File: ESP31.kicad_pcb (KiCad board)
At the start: 4 copper layers, 20.7 x 37.3 mm, 51 parts, among them J1 Conn_01x01, J25 Conn_01x01, J26 Conn_01x01, J27 Conn_01x01, J28 Conn_01x01, J29 Conn_01x01, J30 Conn_01x01, J31 Conn_01x01, J32 Conn_01x01, J33 Conn_01x01, J34 Conn_01x01, J35 Conn_01x01, J36 Conn_01x01, J40 Conn_01x01, J41 Conn_01x01, J42 Conn_01x01, J43 Conn_01x01, J44 Conn_01x01, J45 Conn_01x01, J46 Conn_01x01, J47 Conn_01x01, J48 Conn_01x01, J49 Conn_01x01, J50 Conn_01x01, J51 Conn_01x01, J52 Conn_01x01, J53 Conn_01x01, J54 Conn_01x01, J55 Conn_01x01, J56 Conn_01x01, J57 Conn_01x01, J58 Conn_01x01, J59 Conn_01x01, J60 Conn_01x01, J61 Conn_01x01, J62 Conn_01x01, J63 Conn_01x01, SW1 SW_Push, SW2 SW_Push, U1 ESP32-PICO-D4

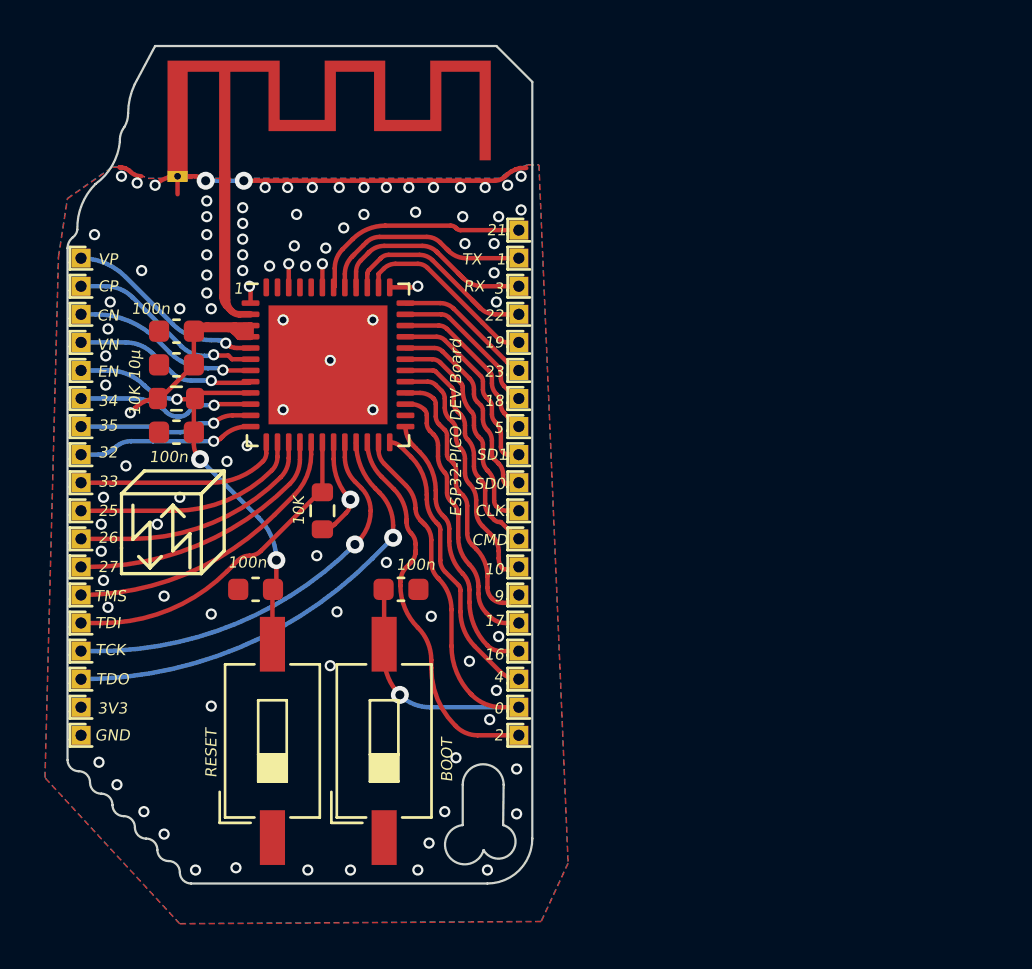
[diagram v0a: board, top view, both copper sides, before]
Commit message: Final Version
Last ordered version. It's working :)
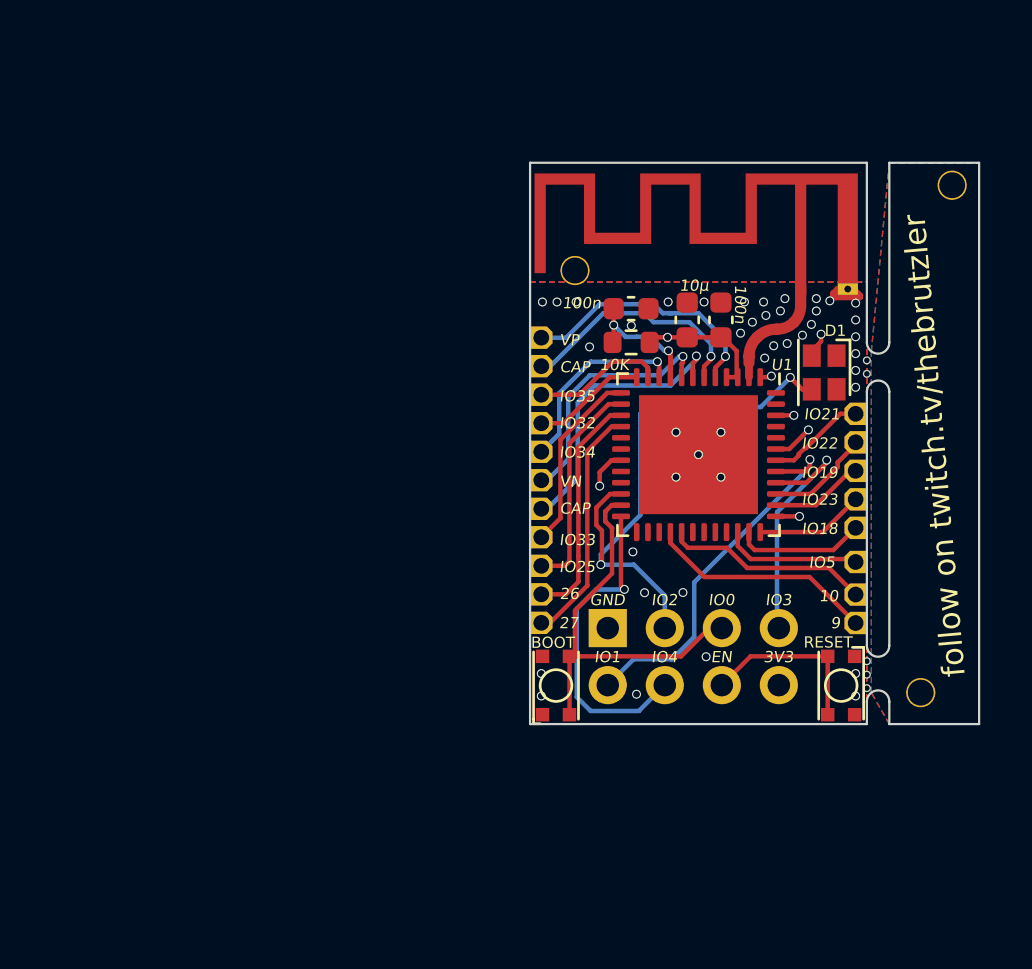
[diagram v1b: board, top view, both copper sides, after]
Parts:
- removed C4, C5: 100n, Capacitor_SMD:C_0603_1608Metric
- removed G***: LOGO, TheBrutzlers_Lib:Platinenmacher_14
- removed J25, J26, J27, J28, J29, J30, J31, J32, J33, J34, J35, J36, J40, J41, J42, J43, J44, J45, J46, J47, J48, J49, J50, J51, J52, J53, J54, J55, J56, J57, J58, J59, J60, J61, J62, J63: Conn_01x01, Connector_PinHeader_1.00mm:PinHeader_1x01_P1.00mm_Vertical
- removed R2: 10K, Resistor_SMD:R_0603_1608Metric
- removed the SM3 at (85.8, 108.3)
- added ?: , , F.Cu at (119.0, 112.2)
- added ?: , , F.Cu at (122.8, 91.0)
- added ?: , , F.Cu at (119.0, 98.8)
- added ?: , , F.Cu at (121.4, 113.6)
- added ?: , , F.Cu at (119.0, 113.4)
- added ?: , , F.Cu at (119.0, 98.6)
- added ?: , , F.Cu at (119.0, 112.8)
- added D1: WS2812B_Geaendertes_Symbol, LED_SMD:LED_Cree-PLCC4_2x2mm_CW, F.Cu at (117.1, 99.3)
- added J10: Conn_01x01, Eigene:CON_1x01, F.Cu at (118.5, 107.8)
- added J11: Conn_01x01, Eigene:CON_1x01, F.Cu at (118.5, 110.5)
- added J12: Conn_01x01, Eigene:CON_1x01, F.Cu at (118.5, 109.2)
- added J13: Conn_01x01, Eigene:CON_1x01, F.Cu at (118.5, 106.3)
- added J14: Conn_01x01, Eigene:CON_1x01, F.Cu at (118.5, 103.7)
- added J15: Conn_01x01, Eigene:CON_1x01, F.Cu at (118.5, 101.2)
- added J16: Conn_01x01, Eigene:CON_1x01, F.Cu at (118.5, 102.5)
- added J17: Conn_01x01, Eigene:CON_1x01, F.Cu at (118.5, 105.0)
- added J18: Conn_01x01, Eigene:CON_1x01, F.Cu at (104.5, 108.0)
- added J19: Conn_01x01, Eigene:CON_1x01, F.Cu at (104.5, 109.2)
- added J20: Conn_01x01, Eigene:CON_1x01, F.Cu at (104.5, 110.5)
- added J21: Conn_01x01, Eigene:CON_1x01, F.Cu at (104.5, 101.6)
- added J22: Conn_01x01, Eigene:CON_1x01, F.Cu at (104.5, 106.7)
- added J23: Conn_01x01, Eigene:CON_1x01, F.Cu at (104.5, 102.9)
- added J24: Conn_01x01, Eigene:CON_1x01, F.Cu at (104.5, 100.3)
- added J3: Conn_01x01, Eigene:CON_1x01, F.Cu at (104.5, 97.8)
- added J4: Conn_01x01, Eigene:CON_1x01, F.Cu at (104.5, 99.1)
- added J5: Conn_01x01, Eigene:CON_1x01, F.Cu at (104.5, 105.4)
- added J6: Conn_01x01, Eigene:CON_1x01, F.Cu at (104.5, 104.1)
- added J8: Conn_01x01, Eigene:CON_1x01, F.Cu at (118.5, 106.7)
- added J9: Conn_01x01, Eigene:CON_1x01, F.Cu at (118.5, 105.4)
- added REF**: jlc_tooling, TheBrutzlers_Lib:jlc_tooling, F.Cu at (106.0, 94.8)
- added REF**: mousebite, TheBrutzlers_Lib:mousebite, F.Cu at (119.0, 99.4)
- AE1: footprint RF_Antenna:Texas_SWRA117D_2.4GHz_Right -> RF_Antenna:Texas_SWRA117D_2.4GHz_Left
- J1: value Conn_01x01 -> Conn_02x04_Odd_Even; footprint Connector_PinHeader_1.00mm:PinHeader_1x01_P1.00mm_Vertical -> Connector_PinHeader_2.54mm:PinHeader_2x04_P2.54mm_Vertical; moved to B.Cu
- SW1, SW2: footprint Button_Switch_SMD:SW_DIP_SPSTx01_Slide_6.7x4.1mm_W8.61mm_P2.54mm_LowProfile -> TheBrutzlers_Lib:microswitch
- moved AE1 26.1 mm to (116.0, 95.6)
- moved SW1 25.5 mm to (117.9, 113.3), turned to -90 degrees
- moved C3 24.3 mm to (112.5, 97.0), turned to -90 degrees
- moved J1 23.9 mm to (107.5, 110.7), turned to -90 degrees
- moved C2 22.8 mm to (111.0, 97.0), turned to -90 degrees
- moved C1 20.9 mm to (108.5, 96.5), turned to 0 degrees
- moved R1 20.4 mm to (108.5, 98.0), turned to 180 degrees
- moved U1 17.0 mm to (111.5, 103.0), turned to -90 degrees
- moved SM3 12.1 mm to (113.2, 103.8)
- moved SW2 8.04 mm to (105.2, 113.3)
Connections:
- U1 pad 17: /MTMS -> unconnected-(U1-Pad17)
- U1 pad 18: /MTDI -> unconnected-(U1-Pad18)
- U1 pad 20: /MTCK -> unconnected-(U1-Pad20)
- U1 pad 21: /MTDO -> unconnected-(U1-Pad21)
- U1 pad 25: Net-(J25-Pad1) -> unconnected-(U1-Pad25)
- U1 pad 27: /IO17 -> unconnected-(U1-Pad27)
- U1 pad 30: /CMD -> unconnected-(U1-Pad30)
- U1 pad 31: Net-(U1-Pad31) -> unconnected-(U1-Pad31)
- U1 pad 32: /SD0 -> unconnected-(U1-Pad32)
- U1 pad 33: /SD1 -> unconnected-(U1-Pad33)
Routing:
- net /MTDO: track 20.5 -> 0.00 mm, vias 1 -> 0
- net /MTCK: track 18.5 -> 0.00 mm, vias 1 -> 0
- net /EN: track 20.3 -> 37.9 mm, vias 3 -> 2
- net /MTDI: track 14.9 -> 0.00 mm
- net GND: track 18.7 -> 4.25 mm, vias 93 -> 42
- net /MTMS: track 13.3 -> 0.00 mm
- net /IO17: track 12.3 -> 0.00 mm
- net Net-(J25-Pad1): track 12.2 -> 0.00 mm
- net /CMD: track 10.2 -> 0.00 mm
- net Net-(U1-Pad31): track 9.83 -> 0.00 mm
- net /SD0: track 9.16 -> 0.00 mm
- net /SD1: track 8.46 -> 0.00 mm
- net +3V3: track 21.4 -> 13.1 mm, vias 6 -> 7
- net Net-(AE1-Pad1): track 13.1 -> 5.23 mm
- net /IO2: track 17.4 -> 24.9 mm, vias 0 -> 2
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- added copper zone on B.Cu, net (none)
- added copper zone on F.Cu, net (none)
- added copper zone on In1.Cu, net (none)
- added copper zone on In2.Cu, net (none)
- added copper zone on B.Cu, net GND
- removed copper zone on B.Cu, net +3V3
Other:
- board size 20.7 x 37.3 mm -> 20 x 25 mm
- board text added: "CAP"
- board text added: "IO0"
- board text added: "IO1"
- board text added: "IO18"
- board text added: "IO19"
- board text added: "IO2"
- board text added: "IO21"
- board text added: "IO22"
- board text added: "IO23"
- board text added: "IO25"
- board text added: "IO3"
- board text added: "IO32"
- board text added: "IO33"
- board text added: "IO34"
- board text added: "IO35"
- board text added: "IO4"
- board text added: "IO5"
- board text added: "U1"
- board text added: "follow on twitch.tv/thebrutzler"
- board text added: "thebrutzler"
- board text removed: "0"
- board text removed: "1"
- board text removed: "16"
- board text removed: "17"
- board text removed: "18"
- board text removed: "19"
- board text removed: "2"
- board text removed: "21"
- board text removed: "22"
- board text removed: "23"
- board text removed: "25"
- board text removed: "3"
- board text removed: "32"
- board text removed: "33"
- board text removed: "34"
- board text removed: "35"
- board text removed: "4"
- board text removed: "5"
- board text removed: "CLK"
- board text removed: "CMD"
- board text removed: "CN"
- board text removed: "CP"
- board text removed: "ESP32-PICO DEV Board"
- board text removed: "RX"
- board text removed: "SD0"
- board text removed: "SD1"
- board text removed: "TCK"
- board text removed: "TDI"
- board text removed: "TDO"
- board text removed: "TMS"
- board text removed: "TX"
